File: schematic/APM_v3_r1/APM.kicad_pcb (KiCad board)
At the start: 4 copper layers, 72.5 x 104.5 mm, 97 parts, among them J1 ACM_CTRL, J11 DAC_L_PRB, J12 Conn_01x02, J13 Conn_02x36_Odd_Even, J14 ADC FFC, J15 FPGA FFC, J16 USB_A, J17 MIDI_DGB, J18 Conn_02x36_Odd_Even, J2 CAN, J29 USB_A, J3 7SDD_CTRL, J30 UART_DEBUG, J4 LCD_display, J5 INTRPT, J7 DAC_R_PRB, U1 NUCLEO-H753ZI, U13 INA219AxD, U2 CH340G, U3 LT1963AxST-3.3, U38 CH340G, U4 W25Q128JVS, U5 MR25H40, U7 INA219AxD, U8 24LC1025-I_P, Y1 12MHz, Y7 12MHz

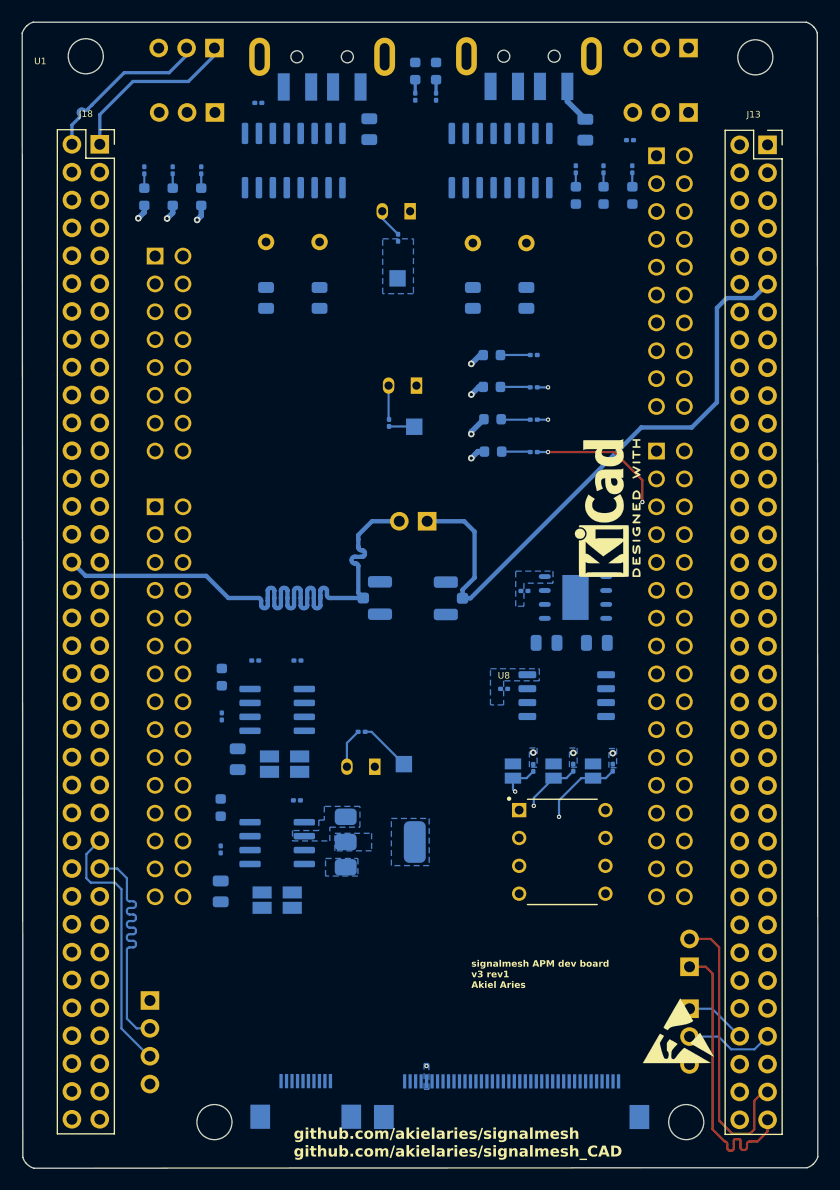
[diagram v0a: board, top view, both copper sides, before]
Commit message: i got orientation wrong big time
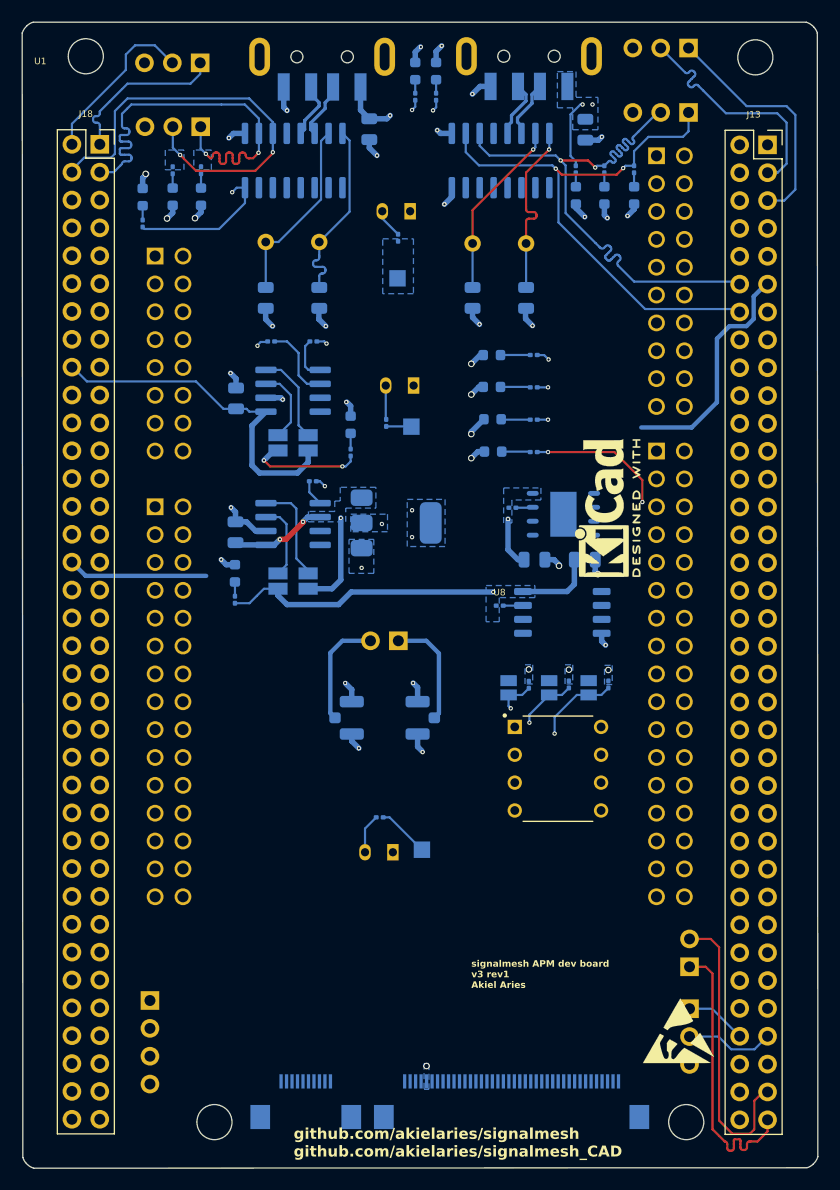
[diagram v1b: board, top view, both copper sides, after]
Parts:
- removed R11, R90: 1k5, Resistor_SMD:R_0201_0603Metric
- R89: value 300 -> 1.2k
- moved G*** 42.4 mm to (84.0, 137.2)
- moved REF** 42.4 mm to (83.2, 139.9)
- moved C5 32.9 mm to (80.0, 85.8)
- moved C7 32.8 mm to (79.9, 98.0)
- moved R3 29.3 mm to (85.2, 89.8)
- moved R16 29.1 mm to (85.2, 102.4)
- moved R26 29.1 mm to (83.2, 80.6)
- moved R28 29.1 mm to (87.0, 80.6)
- moved R4 29.1 mm to (87.0, 93.3)
- moved U13 29.1 mm to (85.2, 85.1)
- moved U3 29.1 mm to (94.5, 97.1)
- moved U7 29.1 mm to (85.2, 97.2)
- moved R30 26.8 mm to (90.4, 90.7)
- moved D7 25.8 mm to (90.4, 88.2)
- moved R15 22.8 mm to (79.8, 104.1)
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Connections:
- J13 pad 12: /APM_USB_D- -> /APM_MIDI_RX
- J13 pad 14: /APM_USB_D+ -> /APM_MIDI_TX
- J13 pad 20: unconnected-(J13-Pin_20-Pad20) -> GND
- J13 pad 21: unconnected-(J13-Pin_21-Pad21) -> /APM_EEPROM_EN
- J13 pad 23: unconnected-(J13-Pin_23-Pad23) -> /APM_MRAM_EN
- J13 pad 25: unconnected-(J13-Pin_25-Pad25) -> /APM_SPIFLASH_EN
- J13 pad 27: unconnected-(J13-Pin_27-Pad27) -> /APM_SPI1_MISO
- J13 pad 29: unconnected-(J13-Pin_29-Pad29) -> /APM_SPI1_MOSI
- J13 pad 31: unconnected-(J13-Pin_31-Pad31) -> /APM_SPI1_SCK
- J13 pad 32: unconnected-(J13-Pin_32-Pad32) -> GND
- J13 pad 33: unconnected-(J13-Pin_33-Pad33) -> /SPIFLASH_CS
- J13 pad 35: unconnected-(J13-Pin_35-Pad35) -> /SPIMRAM_CS
- J13 pad 39: unconnected-(J13-Pin_39-Pad39) -> GND
- J14 pad 9: /3V3_APM -> 3V3_APM
- J17 pad 1: /USB_MIDI_APM/APM_MIDI_TX -> /APM_MIDI_TX
- J17 pad 2: /APM_MIDI_TX -> /APM_MIDI_RX
- J18 pad 47: /APM_SPI1_MOSI -> unconnected-(J18-Pin_47-Pad47)
- J18 pad 57: /APM_MIDI_RX -> unconnected-(J18-Pin_57-Pad57)
- J18 pad 59: /APM_MIDI_TX -> unconnected-(J18-Pin_59-Pad59)
- J18 pad 64: /APM_SPIFLASH_EN -> unconnected-(J18-Pin_64-Pad64)
- J18 pad 65: /APM_SPI1_MISO -> unconnected-(J18-Pin_65-Pad65)
- J18 pad 66: /APM_MRAM_EN -> unconnected-(J18-Pin_66-Pad66)
- J18 pad 68: /APM_EEPROM_EN -> unconnected-(J18-Pin_68-Pad68)
- J18 pad 69: /SPIFLASH_CS -> unconnected-(J18-Pin_69-Pad69)
- J18 pad 71: /SPIMRAM_CS -> unconnected-(J18-Pin_71-Pad71)
- J18 pad 72: /APM_SPI1_SCK -> unconnected-(J18-Pin_72-Pad72)
- J30 pad 1: /USB_debug_APM/APM_DBG_TX -> /APM_DBG_TX
- J30 pad 2: /APM_DBG_TX -> /APM_DBG_RX
- R12 pad 1: /APM_MIDI_RX -> /APM_MIDI_TX
- R13 pad 1: /APM_MIDI_TX -> /APM_MIDI_RX
- R15 pad 2: /3V3_APM -> 3V3_APM
- R16 pad 4: /3V3_APM -> 3V3_APM
- R91 pad 1: /APM_DBG_RX -> /APM_DBG_TX
- R92 pad 1: /APM_DBG_TX -> /APM_DBG_RX
- U2 pad 2: /APM_MIDI_RX -> /APM_MIDI_TX
- U2 pad 3: /APM_MIDI_TX -> /APM_MIDI_RX
- U38 pad 2: /APM_DBG_RX -> /APM_DBG_TX
- U38 pad 3: /APM_DBG_TX -> /APM_DBG_RX
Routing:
- net /APM_MIDI_TX: track 0.00 -> 51.9 mm, vias 0 -> 2
- net /APM_MIDI_RX: track 0.00 -> 51.7 mm, vias 0 -> 2
- net GND: track 10.4 -> 60.3 mm, vias 11 -> 44
- net /APM_DBG_RX: track 0.00 -> 39.8 mm, vias 0 -> 2
- net /APM_DBG_TX: track 0.00 -> 39.5 mm, vias 0 -> 2
- net 3V3_APM: track 0.00 -> 37.4 mm, vias 0 -> 2
- net 5V_APM: track 3.68 -> 40.2 mm, vias 0 -> 11
- net /DAC_1-1_R: track 55.7 -> 23.0 mm
- net 5V_APM_MCU: track 0.00 -> 31.7 mm
- net /DAC_1-2_L: track 56.0 -> 31.8 mm
- net /APM_I2C2_SCL: track 23.9 -> 0.00 mm
- net /APM_I2C2_SDA: track 22.8 -> 0.00 mm
- net /APM_CAN_TD: track 0.00 -> 22.0 mm
- net /APM_CAN_RD: track 0.00 -> 21.9 mm
- net 3V3_LDO: track 0.00 -> 17.9 mm, vias 0 -> 3
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- added copper zone on B.Cu, net /APM_DBG_RX
- added copper zone on B.Cu, net /APM_DBG_TX
